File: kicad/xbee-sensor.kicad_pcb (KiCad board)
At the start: 2 copper layers, 44 x 60 mm, 37 parts, among them J1 Solar, J2 I2C, J3 Battery, J4 PIR, J5 SWD, Q1 NX2301P, Q2 NX2301P, SW1 RESET, SW2 BOOT0, U1 LD1117S33TR_SOT223, U2 MCP73831-2-OT, U3 XBee_Module_TH, U4 STM32L031K6Tx, U5 A3213EUA-T, Y1 Crystal

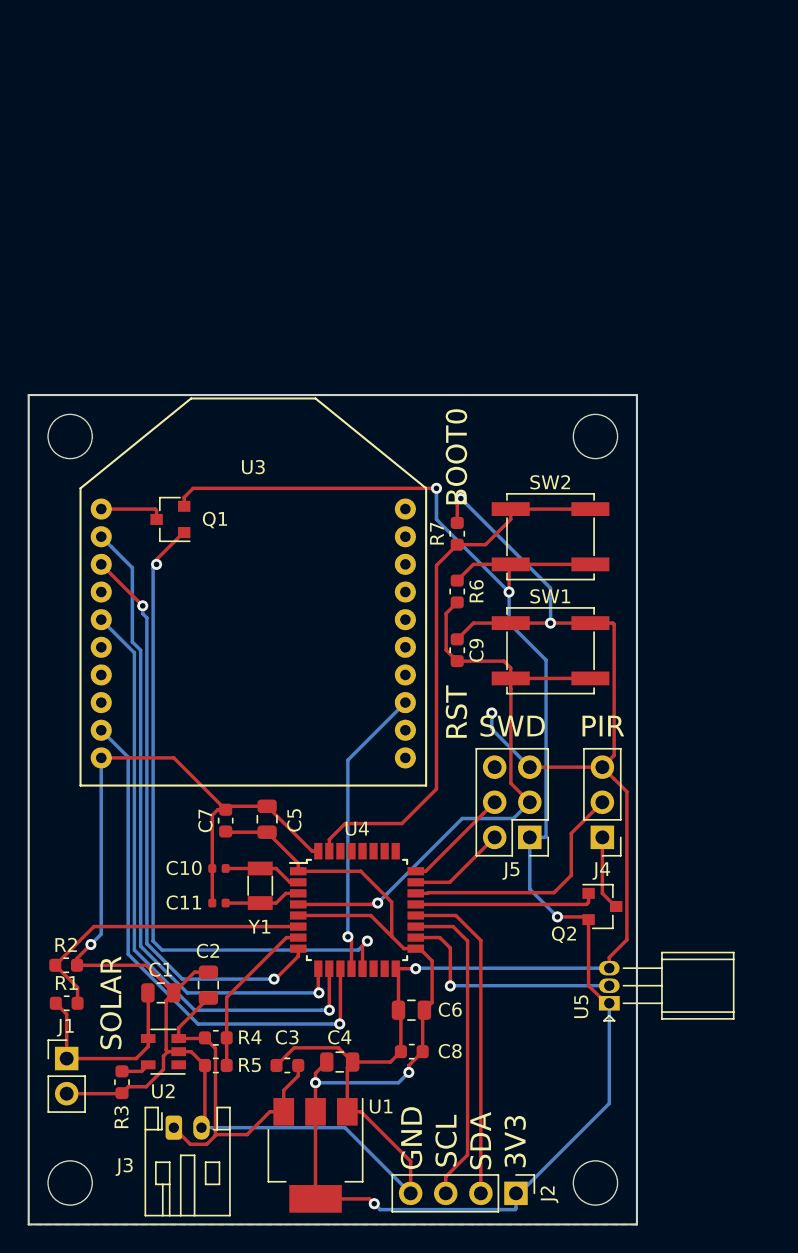
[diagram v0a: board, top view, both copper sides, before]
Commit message: Version 2.0 layout
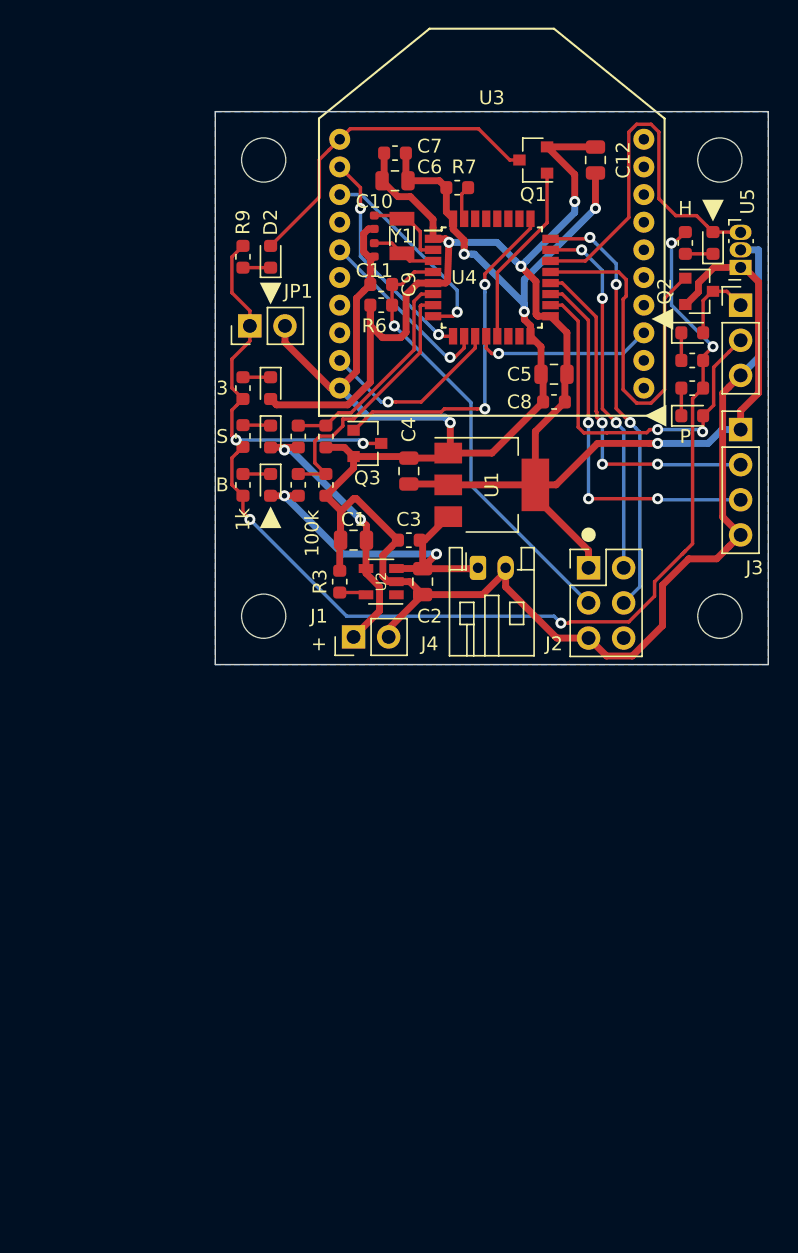
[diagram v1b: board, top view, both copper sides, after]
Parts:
- removed the REF** at (149.5, 98.5)
- removed the REF** at (111.5, 98.5)
- removed the REF** at (111.5, 152.5)
- removed the REF** at (149.5, 152.5)
- removed SW1: RESET, Button_Switch_SMD:SW_SPST_EVPBF
- removed SW2: BOOT0, Button_Switch_SMD:SW_SPST_EVPBF
- added C12: 10uF, Capacitor_SMD:C_0805_2012Metric, F.Cu at (149.5, 78.5)
- added D1: LED, LED_SMD:LED_0603_1608Metric, F.Cu at (156.5, 91.0)
- added D2: LED, LED_SMD:LED_0603_1608Metric, F.Cu at (126.0, 85.5)
- added D3: LED, LED_SMD:LED_0603_1608Metric, F.Cu at (158.0, 84.5)
- added D4: LED, LED_SMD:LED_0603_1608Metric, F.Cu at (156.5, 97.0)
- added D5: LED, LED_SMD:LED_0603_1608Metric, F.Cu at (126.0, 98.5)
- added D6: LED, LED_SMD:LED_0603_1608Metric, F.Cu at (126.0, 102.0)
- added D7: LED, LED_SMD:LED_0603_1608Metric, F.Cu at (126.0, 95.0)
- added JP1: LED_EN, Connector_PinHeader_2.54mm:PinHeader_1x02_P2.54mm_Vertical, F.Cu at (124.5, 90.5)
- added Q3: SI2333DDS, Package_TO_SOT_SMD:SOT-23, F.Cu at (133.0, 99.0)
- added R10: 1k, Resistor_SMD:R_0603_1608Metric, F.Cu at (156.0, 84.5)
- added R11: 1k, Resistor_SMD:R_0603_1608Metric, F.Cu at (156.5, 95.0)
- added R12: 1k, Resistor_SMD:R_0603_1608Metric, F.Cu at (124.0, 98.5)
- added R13: 1k, Resistor_SMD:R_0603_1608Metric, F.Cu at (124.0, 102.0)
- added R14: 1k, Resistor_SMD:R_0603_1608Metric, F.Cu at (124.0, 95.0)
- added R8: 1k, Resistor_SMD:R_0603_1608Metric, F.Cu at (156.5, 93.0)
- added R9: 1k, Resistor_SMD:R_0603_1608Metric, F.Cu at (124.0, 85.5)
- added REF**: MountingHole_3.2mm_M3_ISO14580, MountingHole:MountingHole_3.2mm_M3_ISO14580, F.Cu at (158.5, 78.5)
- added REF**: MountingHole_3.2mm_M3_ISO14580, MountingHole:MountingHole_3.2mm_M3_ISO14580, F.Cu at (125.5, 78.5)
- added REF**: MountingHole_3.2mm_M3_ISO14580, MountingHole:MountingHole_3.2mm_M3_ISO14580, F.Cu at (125.5, 111.5)
- added REF**: MountingHole_3.2mm_M3_ISO14580, MountingHole:MountingHole_3.2mm_M3_ISO14580, F.Cu at (158.5, 111.5)
- J2: value I2C -> SWD; footprint Connector_PinHeader_2.54mm:PinHeader_1x04_P2.54mm_Vertical -> Connector_PinHeader_2.54mm:PinHeader_2x03_P2.54mm_Vertical
- J3: value Battery -> I2C; footprint Connector_JST:JST_PH_S2B-PH-K_1x02_P2.00mm_Horizontal -> Connector_PinHeader_2.54mm:PinHeader_1x04_P2.54mm_Vertical
- J4: value PIR -> Battery; footprint Connector_PinHeader_2.54mm:PinHeader_1x03_P2.54mm_Vertical -> Connector_JST:JST_PH_S2B-PH-K_1x02_P2.00mm_Horizontal
- J5: value SWD -> PIR; footprint Connector_PinHeader_2.54mm:PinHeader_2x03_P2.54mm_Vertical -> Connector_PinHeader_2.54mm:PinHeader_1x03_P2.54mm_Vertical
- U5: value A3213EUA-T -> A3213; footprint Package_TO_SOT_THT:TO-92_Inline_W4.0mm_Horizontal_FlatSideDown -> Sensor_Current:Allegro_SIP-3
- moved J3 65.0 mm to (160.0, 98.0)
- moved C6 60.0 mm to (135.0, 80.0), turned to 0 degrees
- moved U5 54.1 mm to (160.0, 86.3)
- moved U1 50.1 mm to (142.0, 102.0), turned to 0 degrees
- moved C7 49.8 mm to (135.0, 78.0), turned to 0 degrees
- moved C11 48.6 mm to (133.5, 85.0), turned to 270 degrees
- moved C8 48.1 mm to (146.5, 96.0)
- moved Y1 48.1 mm to (135.5, 84.0)
- moved C10 48.1 mm to (133.5, 83.0), turned to 90 degrees
- moved U4 46.8 mm to (142.0, 87.0)
- moved J2 45.6 mm to (149.0, 108.0), turned to 0 degrees
- moved Q2 45.0 mm to (157.0, 88.0)
- moved R1 44.3 mm to (128.0, 98.5), turned to 90 degrees
- moved C4 43.0 mm to (136.0, 101.0), turned to 90 degrees
- moved R5 42.7 mm to (130.0, 102.0), turned to 270 degrees
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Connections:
- net Net-(Q1-Pad3) renamed XBEE_PWR
- J2 pad 2: I2C_SDA -> SWDIO
- J2 pad 3: I2C_SCL -> NRST
- J2 pad 4: GND -> SWCLK
- J3 pad 1: BATTERY -> +3V3
- J3 pad 2: GND -> I2C_SDA
- J4 pad 1: Net-(J4-Pad1) -> BATTERY
- J4 pad 2: PIR -> GND
- J5 pad 1: +3V3 -> PIR_PWR
- J5 pad 2: SWDIO -> PIR
- J5 pad 3: NRST -> GND
- Q2 pad 3: Net-(J4-Pad1) -> PIR_PWR
- U4 pad 18: HALL -> PIR
- U4 pad 22: PIR -> HALL
- U4 pad 25: Net-(U4-Pad25) -> ~LED_EN
- U5 pad 2: HALL -> GND
- U5 pad 3: GND -> HALL
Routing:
- net LED_GND: track 0.00 -> 97.0 mm, vias 0 -> 6
- net BOOT0: track 39.5 -> 2.51 mm
- net +3V3: track 163.4 -> 127.1 mm, vias 6 -> 4
- net EN_XBEE: track 48.7 -> 13.3 mm, vias 2 -> 0
- net XB_RX: track 46.9 -> 16.2 mm, vias 1 -> 2
- net XB_RESET: track 43.8 -> 13.4 mm
- net GND: track 198.0 -> 169.6 mm, vias 5 -> 4
- net XB_TX: track 42.0 -> 14.8 mm, vias 2 -> 1
- net ~LED_EN: track 0.00 -> 25.3 mm, vias 0 -> 2
- net XB_SLEEP_REQ: track 38.4 -> 13.5 mm
- net SWCLK: track 7.78 -> 31.3 mm, vias 0 -> 3
- net SWDIO: track 7.06 -> 26.5 mm, vias 0 -> 3
- net XBEE_PWR: track 4.69 -> 24.0 mm
- net EN_PIR: track 13.2 -> 26.3 mm
- net NRST: track 45.1 -> 32.3 mm
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- removed copper zone on F.Cu, net GND
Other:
- board size 44 x 60 mm -> 40 x 40 mm
- net class Power added: clearance 0.2, trace_width 0.5, via_dia 0.8, via_drill 0.4
- rule pad_to_mask_clearance: 0.051 -> 0
- rule solder_mask_min_width: 0.1 -> 0.25
- board text added: "+"
- board text added: "100k"
- board text added: "1k"
- board text added: "3"
- board text added: "B"
- board text added: "CLK"
- board text added: "H"
- board text added: "HALL"
- board text added: "NRST"
- board text added: "P"
- board text added: "PWR"
- board text added: "S"
- board text added: "SWDIO"
- board text added: "v@nce.me XBee Sensor V2.0"
- board text added: "▼"
- board text added: "●"
- board text removed: "BOOT0"
- board text removed: "RST"
- board text removed: "SWD"
- board text removed: "v@nce.me XBee Sensor V1.0"

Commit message: Created V2 ready for manufacture
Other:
- rule solder_mask_min_width: 0.25 -> 0.2
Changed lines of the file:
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@@
-(kicad_pcb (version 20171130) (host pcbnew "(5.0.1-3-g963ef8bb5)")
+(kicad_pcb (version 20171130) (host pcbnew 5.0.2-bee76a0~70~ubuntu18.10.1)
   (general
     (thickness 1.6)
-    (drawings 36)
+    (drawings 40)
     (tracks 459)
     (zones 0)
@@
     (pad_drill 3.2)
     (pad_to_mask_clearance 0)
-    (solder_mask_min_width 0.25)
+    (solder_mask_min_width 0.2)
     (aux_axis_origin 0 0)
     (visible_elements FFFDFF7F)
     (pcbplotparams
       (layerselection 0x010fc_ffffffff)
-      (usegerberextensions false)
+      (usegerberextensions true)
       (usegerberattributes false)
       (usegerberadvancedattributes false)
@@
       (outputformat 1)
       (mirror false)
-      (drillshape 1)
+      (drillshape 0)
       (scaleselection 1)
       (outputdirectory ""))
@@
     (descr "LQFP32: plastic low profile quad flat package; 32 leads; body 7 x 7 x 1.4 mm (see NXP sot358-1_po.pdf and sot358-1_fr.pdf)")
     (tags "QFP 0.8")
+    (solder_mask_margin -0.01)
     (attr smd)
     (fp_text reference U4 (at -2 0) (layer F.SilkS)
@@
     (descr "Allegro Microsystems SIP-3, 1.27mm Pitch (http://www.allegromicro.com/~/media/Files/Datasheets/A1369-Datasheet.ashx)")
     (tags "Allegro SIP-3")
+    (solder_mask_margin -0.01)
     (fp_text reference U5 (at 4.77 0.5 90) (layer F.SilkS)
       (effects (font (size 1 1) (thickness 0.15)))
@@
     )
   )
+  (dimension 33.147 (width 0.3) (layer Dwgs.User)
+    (gr_text "33.147 mm" (at 142.0495 122.496) (layer Dwgs.User)
+      (effects (font (size 1.5 1.5) (thickness 0.3)))
+    )
+    (feature1 (pts (xy 158.623 111.506) (xy 158.623 120.982421)))
+    (feature2 (pts (xy 125.476 111.506) (xy 125.476 120.982421)))
+    (crossbar (pts (xy 125.476 120.396) (xy 158.623 120.396)))
+    (arrow1a (pts (xy 158.623 120.396) (xy 157.496496 120.982421)))
+    (arrow1b (pts (xy 158.623 120.396) (xy 157.496496 119.809579)))
+    (arrow2a (pts (xy 125.476 120.396) (xy 126.602504 120.982421)))
+    (arrow2b (pts (xy 125.476 120.396) (xy 126.602504 119.809579)))
+  )
+  (dimension 40.005 (width 0.3) (layer Dwgs.User)
+    (gr_text "40.005 mm" (at 142.0495 128.084) (layer Dwgs.User)
+      (effects (font (size 1.5 1.5) (thickness 0.3)))
+    )
+    (feature1 (pts (xy 162.052 114.935) (xy 162.052 126.570421)))
+    (feature2 (pts (xy 122.047 114.935) (xy 122.047 126.570421)))
+    (crossbar (pts (xy 122.047 125.984) (xy 162.052 125.984)))
+    (arrow1a (pts (xy 162.052 125.984) (xy 160.925496 126.570421)))
+    (arrow1b (pts (xy 162.052 125.984) (xy 160.925496 125.397579)))
+    (arrow2a (pts (xy 122.047 125.984) (xy 123.173504 126.570421)))
+    (arrow2b (pts (xy 122.047 125.984) (xy 123.173504 125.397579)))
+  )
+  (dimension 33.020244 (width 0.3) (layer Dwgs.User)
+    (gr_text "33.020 mm" (at 172.089802 94.94396 270.2203673) (layer Dwgs.User)
+      (effects (font (size 1.5 1.5) (thickness 0.3)))
+    )
+    (feature1 (pts (xy 158.623 111.506) (xy 170.639735 111.459782)))
+    (feature2 (pts (xy 158.496 78.486) (xy 170.512735 78.439782)))
+    (crossbar (pts (xy 169.926318 78.442037) (xy 170.053318 111.462037)))
+    (arrow1a (pts (xy 170.053318 111.462037) (xy 169.462569 110.337797)))
+    (arrow1b (pts (xy 170.053318 111.462037) (xy 170.635402 110.333286)))
+    (arrow2a (pts (xy 169.926318 78.442037) (xy 169.344234 79.570788)))
+    (arrow2b (pts (xy 169.926318 78.442037) (xy 170.517067 79.566277)))
+  )
+  (dimension 39.878 (width 0.3) (layer Dwgs.User)
+    (gr_text "39.878 mm" (at 179.646 94.996 270) (layer Dwgs.User)
+      (effects (font (size 1.5 1.5) (thickness 0.3)))
+    )
+    (feature1 (pts (xy 162.052 114.935) (xy 178.132421 114.935)))
+    (feature2 (pts (xy 162.052 75.057) (xy 178.132421 75.057)))
+    (crossbar (pts (xy 177.546 75.057) (xy 177.546 114.935)))
+    (arrow1a (pts (xy 177.546 114.935) (xy 176.959579 113.808496)))
+    (arrow1b (pts (xy 177.546 114.935) (xy 178.132421 113.808496)))
+    (arrow2a (pts (xy 177.546 75.057) (xy 176.959579 76.183504)))
+    (arrow2b (pts (xy 177.546 75.057) (xy 178.132421 76.183504)))
+  )
   (gr_text "v@nce.me\nXBee Sensor\nV2.0" (at 142.5 94) (layer B.SilkS)
